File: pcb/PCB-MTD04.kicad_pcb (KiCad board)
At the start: 2 copper layers, 48 parts, among them J1 MotorX, J10 SC_BTNS, J2 Barrel_Jack_Switch, J3 BAU, J4 MotorY, J5 SD, J6 OLED_Screen, J7 SW_XMIN, J8 SW_YMAX, J9 SERVO, SW1 SW_Push, U1 ESP32-S3-UNO, U2 R-78E5.0-1.0

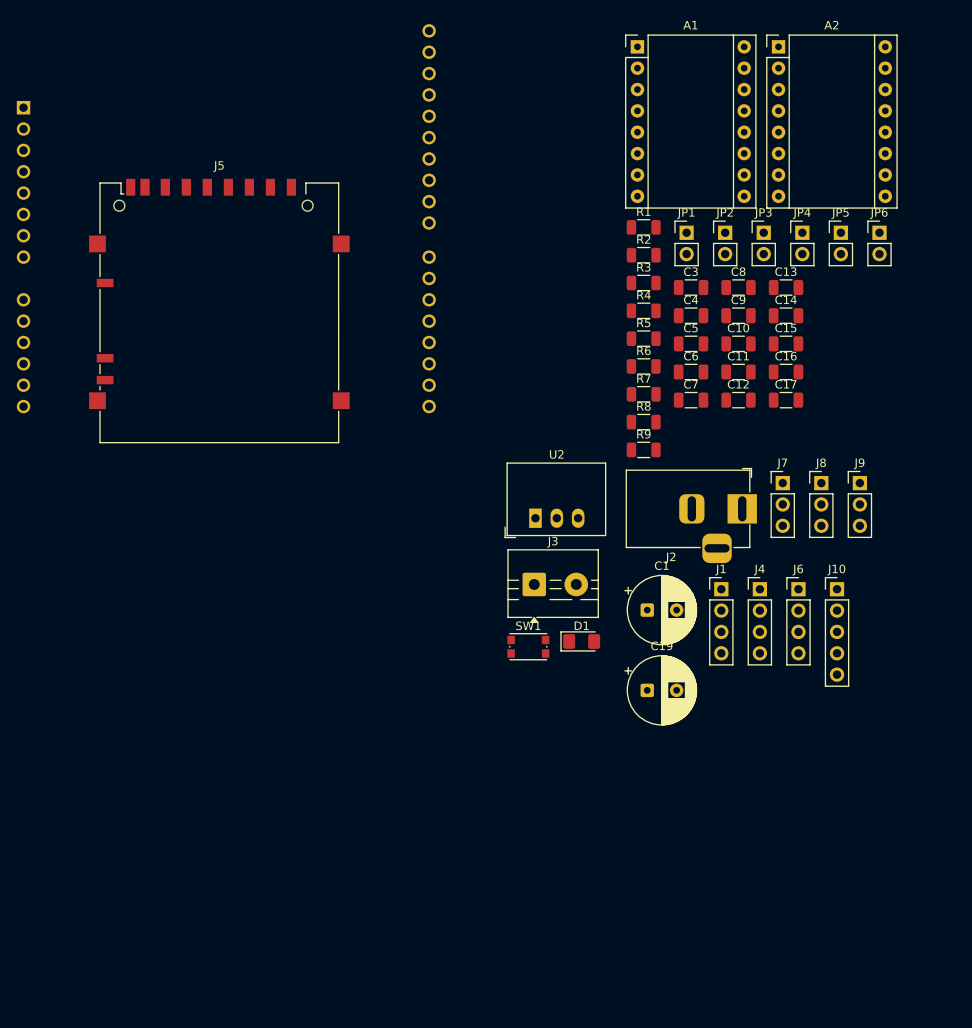
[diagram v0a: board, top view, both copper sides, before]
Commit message: uploadPCB
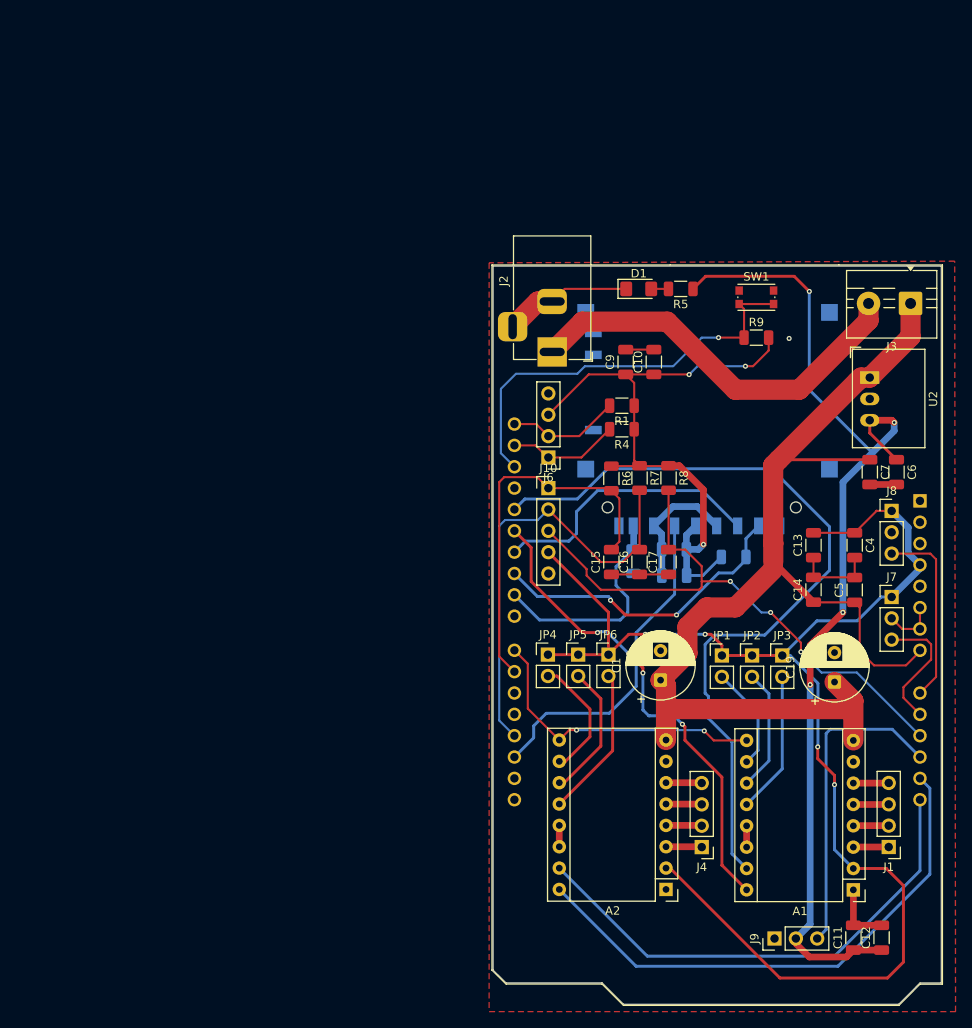
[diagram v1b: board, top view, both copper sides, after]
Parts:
- C3, C8, J5, R2, R3: moved to B.Cu
- moved U1 134.8 mm to (165.9, 142.3), turned to -90 degrees
- moved A1 103.5 mm to (157.9, 153.0), turned to 180 degrees
- moved A2 101.2 mm to (135.7, 153.0), turned to 180 degrees
- moved C11 68.7 mm to (157.9, 158.7), turned to 90 degrees
- moved C12 66.2 mm to (161.3, 158.7), turned to 90 degrees
- moved JP6 59.7 mm to (128.8, 125.0)
- moved JP5 59.1 mm to (125.2, 125.0)
- moved J5 59.0 mm to (140.6, 94.8)
- moved JP4 58.6 mm to (121.6, 125.0)
- moved J3 55.9 mm to (164.8, 83.2), turned to 180 degrees
- moved J9 55.1 mm to (148.6, 158.8), turned to 90 degrees
- moved JP1 50.5 mm to (142.3, 125.1)
- moved JP2 50.4 mm to (145.9, 125.1)
- moved JP3 50.4 mm to (149.5, 125.1)
- moved SW1 49.6 mm to (146.4, 82.5)
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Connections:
- A1 pad 1: +3V3 -> GND
- A1 pad 7: +3V3 -> GND
- A2 pad 1: +3V3 -> GND
- A2 pad 7: +3V3 -> GND
- C1 pad 2: +3V3 -> GND
- C10 pad 2: +3V3 -> GND
- C11 pad 2: +3V3 -> GND
- C12 pad 2: +3V3 -> GND
- C13 pad 1: +3V3 -> GND
- C14 pad 2: +3V3 -> GND
- C15 pad 1: +3V3 -> GND
- C16 pad 1: +3V3 -> GND
- C17 pad 1: +3V3 -> GND
- C19 pad 2: +3V3 -> GND
- C3 pad 2: +3V3 -> GND
- C4 pad 2: +3V3 -> GND
- C5 pad 2: +3V3 -> GND
- C6 pad 2: +3V3 -> GND
- C7 pad 2: +3V3 -> GND
- C8 pad 2: +3V3 -> GND
- C9 pad 2: +3V3 -> GND
- D1 pad 1: +3V3 -> GND
- J10 pad 5: +3V3 -> GND
- J2 pad 1: Net-(J3-Pin_1) -> Net-(J3-Pin_2)
- J2 pad 2: +3V3 -> GND
- J2 pad 3: +3V3 -> GND
- J3 pad 1: Net-(J3-Pin_1) -> +12V
- J3 pad 2: +12V -> Net-(J3-Pin_2)
- J5 pad 3: +3V3 -> GND
- J5 pad 6: +3V3 -> GND
- J6 pad 4: +3V3 -> GND
- J7 pad 2: +3V3 -> GND
- J8 pad 2: +3V3 -> GND
- J9 pad 1: +3V3 -> GND
- SW1 pad 1: +3V3 -> GND
- U1 pad 29: +3V3 -> GND
- U1 pad 6: +3V3 -> GND
- U1 pad 7: +3V3 -> GND
- U2 pad 2: +3V3 -> GND
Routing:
- net +3V3: track 0.00 -> 239.8 mm, vias 0 -> 7
- net +12V: track 0.00 -> 136.0 mm
- net +5V: track 0.00 -> 124.6 mm, vias 0 -> 4
- net /Step-X: track 0.00 -> 94.7 mm
- net /BTN_OK: track 0.00 -> 70.3 mm, vias 0 -> 3
- net GND: track 0.00 -> 68.3 mm
- net /Dir-Y: track 0.00 -> 64.3 mm
- net /Step-Y: track 0.00 -> 59.9 mm
- net /Dir-X: track 0.00 -> 57.8 mm, vias 0 -> 4
- net /BTN_DN: track 0.00 -> 53.5 mm
- net /RST: track 0.00 -> 49.7 mm, vias 0 -> 1
- net Net-(J3-Pin_2): track 0.00 -> 47.9 mm
- net /BTN_UP: track 0.00 -> 45.4 mm
- net /CLK: track 0.00 -> 39.8 mm
- net /SERVO_PWM: track 0.00 -> 37.6 mm
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- added copper zone on F.Cu, net GND
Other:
- board outline added: 53.3 x 87.8 mm
